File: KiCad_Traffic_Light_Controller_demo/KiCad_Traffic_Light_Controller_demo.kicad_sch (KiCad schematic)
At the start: 64 parts, among them J1 Conn_02x08_Odd_Even, J2 Conn_02x08_Odd_Even, J3 Conn_02x05_Odd_Even, J4 +5V, SW1 RST, SW2 OVR, SW3 EN, U1 SM420561N, U2 SM420561N, U3 LM1117DT-3.3

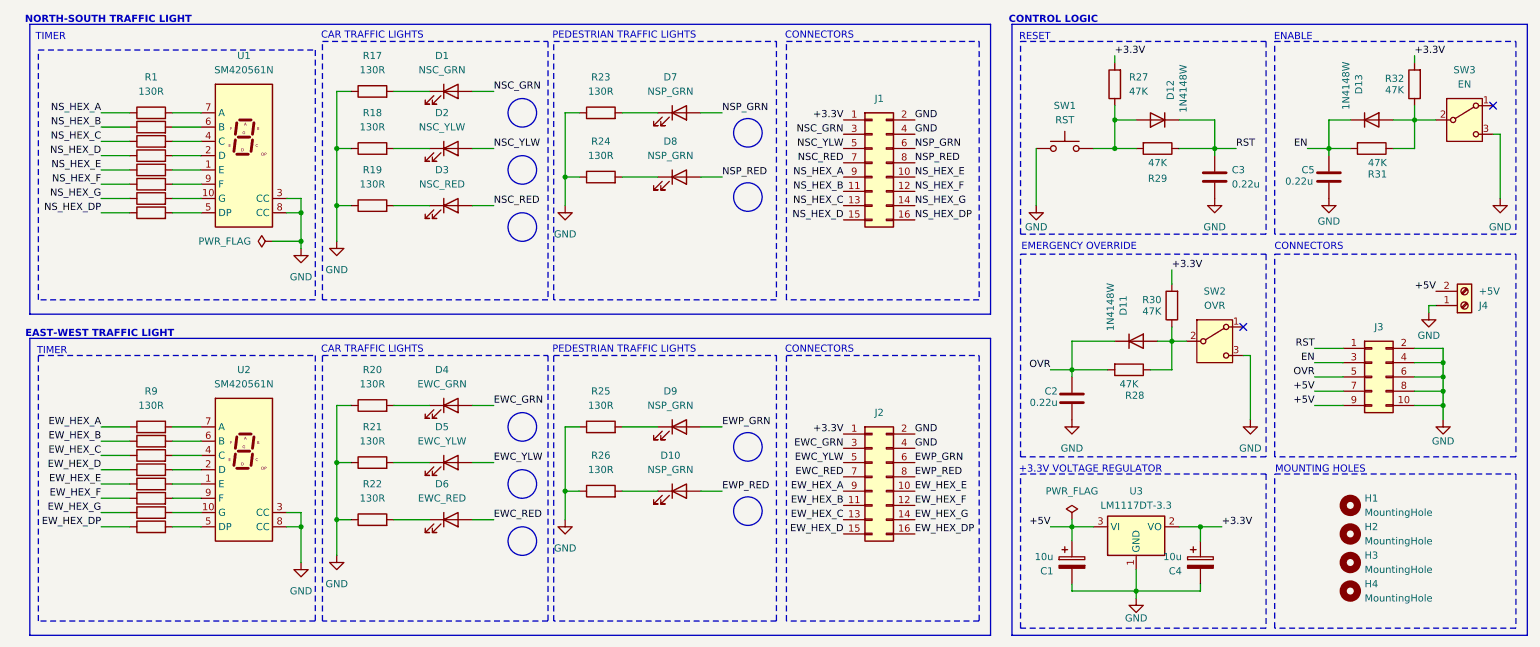
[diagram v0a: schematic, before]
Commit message: Updated KiCad_Traffic_Light_Controller_demo
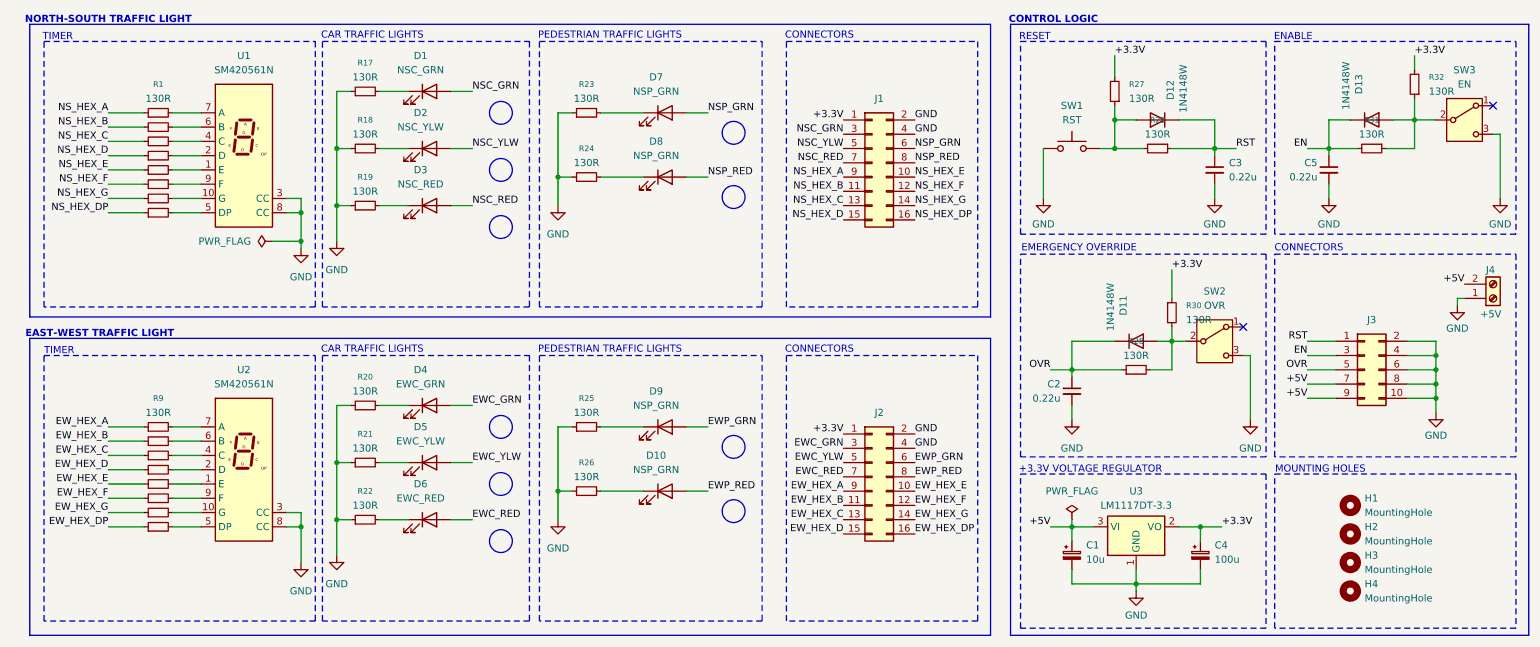
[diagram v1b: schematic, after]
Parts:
- removed C1, C4: 10u, symbol Device:C_Polarized
- removed C2, C3, C5: 0.22u, symbol Device:C
- removed R1, R10, R11, R12, R13, R14, R15, R16, R17, R18, R19, R2, R20, R21, R22, R23, R24, R25, R26, R3, R4, R5, R6, R7, R8, R9: 130R, symbol Device:R
- removed R27, R28, R29, R30, R31, R32: 47K, symbol Device:R
- added C1: 10u, symbol Device:C_Polarized_Small
- added C2, C3, C5: 0.22u, symbol Device:C_Small
- added C4: 100u, symbol Device:C_Polarized_Small
- added R1, R10, R11, R12, R13, R14, R15, R16, R17, R18, R19, R2, R20, R21, R22, R23, R24, R25, R26, R27, R28, R29, R3, R30, R31, R32, R4, R5, R6, R7, R8, R9: 130R, symbol Device:R_Small
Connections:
- net +3.3V: now also C4.1, R27.2, R30.1, R32.2
- net +5V: now also C1.1
- net EN: now also C5.1, R31.2
- net EW_HEX_A: now also R9.1
- net EW_HEX_B: now also R10.1
- net EW_HEX_C: now also R11.1
- net EW_HEX_D: now also R12.1
- net EW_HEX_DP: now also R16.1
- net EW_HEX_E: now also R13.1
- net EW_HEX_F: now also R14.1
- net EW_HEX_G: now also R15.1
- net GND: now also C1.2, C2.2, C3.2, C4.2, C5.2, R17.1, R18.1, R19.1, R20.1, R21.1, R22.1, R23.1, R24.1, R25.1, R26.1
- net NS_HEX_A: now also R1.1
- net NS_HEX_B: now also R2.1
- net NS_HEX_C: now also R3.1
- net NS_HEX_D: now also R4.1
- net NS_HEX_DP: now also R8.1
- net NS_HEX_E: now also R5.1
- net NS_HEX_F: now also R6.1
- net NS_HEX_G: now also R7.1
- net OVR: now also C2.1, R28.1
- net RST: now also C3.1, R29.1
- net at D2.1 (K): now also R18.2
- net at D8.1 (K): now also R24.2
- net at D13.2 (A), SW3.2 (B): now also R31.1, R32.1
- net at D1.1 (K): now also R17.2
- net at D11.2 (A), SW2.2 (B): now also R28.2, R30.2
- net at U2.2 (D): now also R12.2
- net at D12.2 (A), SW1.2: now also R27.1, R29.2
- net at D7.1 (K): now also R23.2
- net at D4.1 (K): now also R20.2
- net at D9.1 (K): now also R25.2
- net at U2.6 (B): now also R10.2
- net at U1.5 (DP): now also R8.2
- net at U2.5 (DP): now also R16.2
- net at D3.1 (K): now also R19.2
- net at D10.1 (K): now also R26.2
- net at U1.1 (E): now also R5.2
- net at U1.10 (G): now also R7.2
- net at U1.2 (D): now also R4.2
- net at U1.4 (C): now also R3.2
- net at U1.6 (B): now also R2.2
- net at U1.7 (A): now also R1.2
- net at U1.9 (F): now also R6.2
- net at U2.7 (A): now also R9.2
- net at U2.10 (G): now also R15.2
- net at D6.1 (K): now also R22.2
- net at U2.4 (C): now also R11.2
- net at U2.1 (E): now also R13.2
- net at U2.9 (F): now also R14.2
- net at D5.1 (K): now also R21.2
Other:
- moved on the sheet: D1, D10, D2, D3, D7, D8, D9, J3, J4, SW1
